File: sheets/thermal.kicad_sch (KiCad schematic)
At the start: 40 parts, among them U1 MAX31856, U3 MAX31856, U4 MAX31856, U5 MAX31856, U6 MAX31856, U7 MAX31856, U8 MAX31856, U9 MAX31856

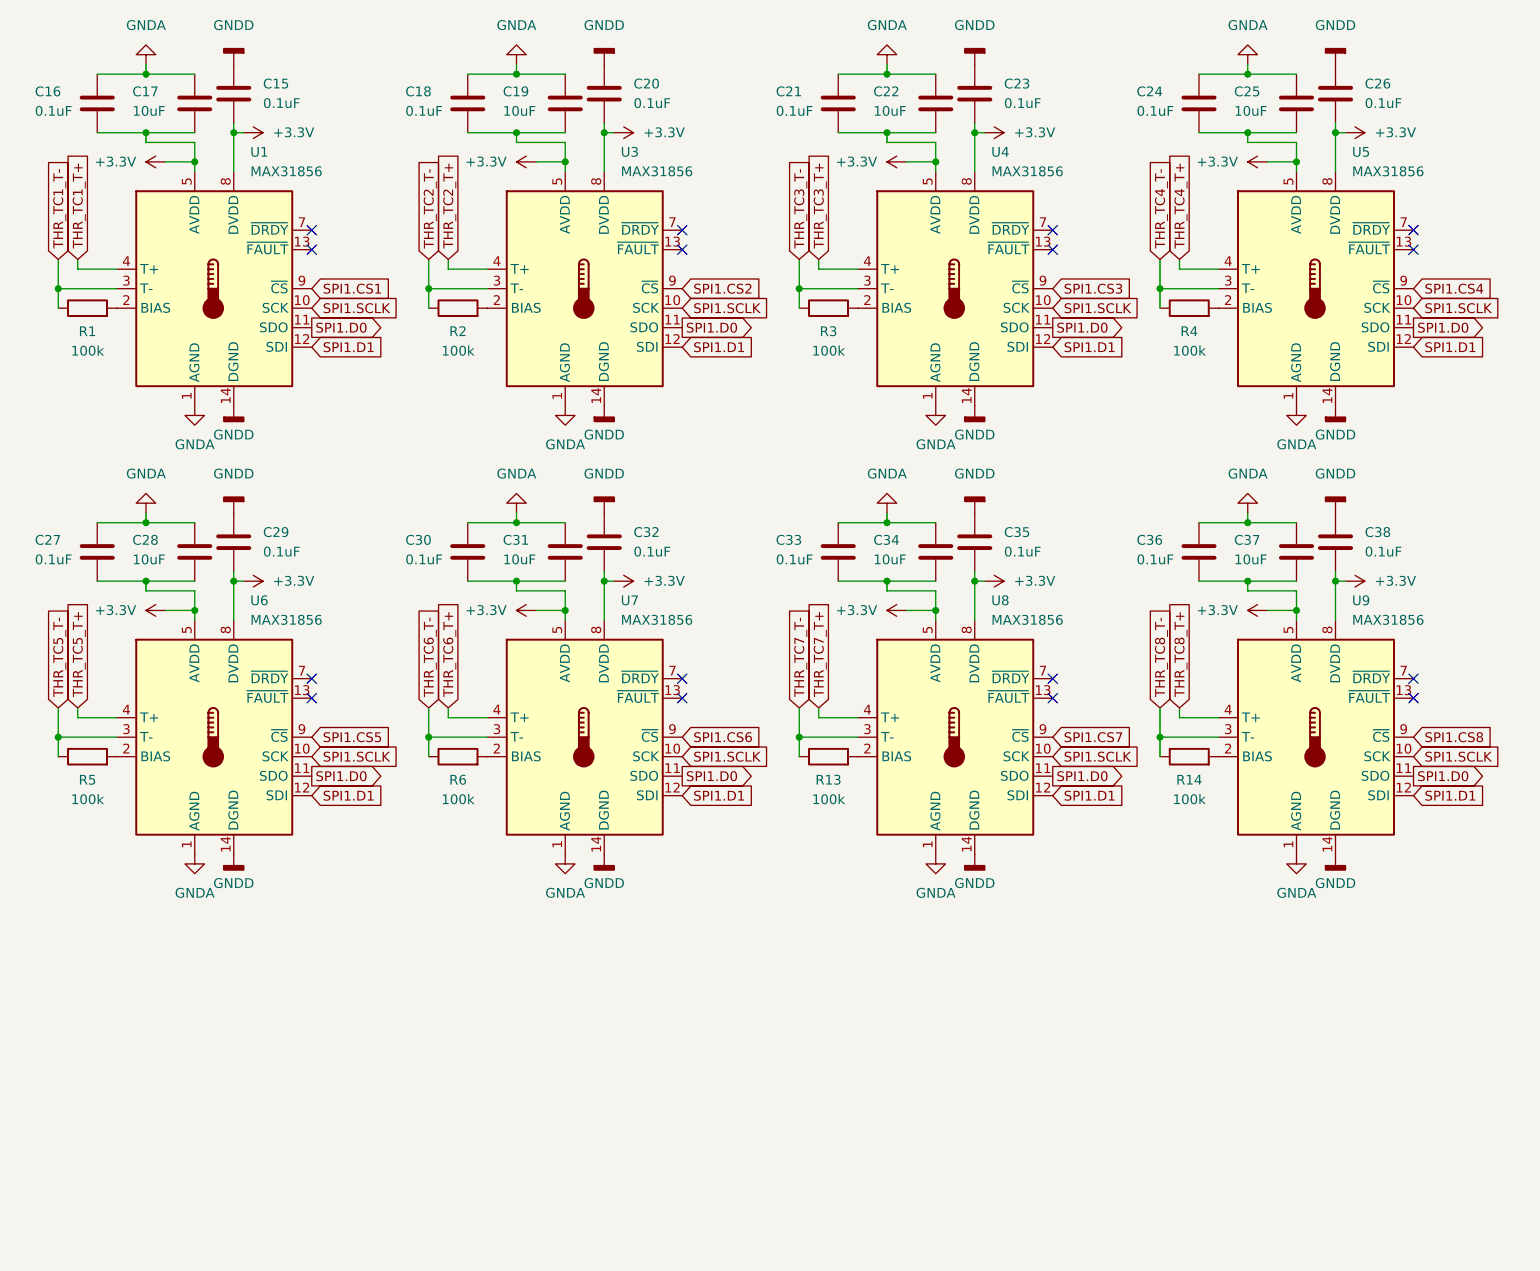
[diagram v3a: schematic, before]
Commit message: push
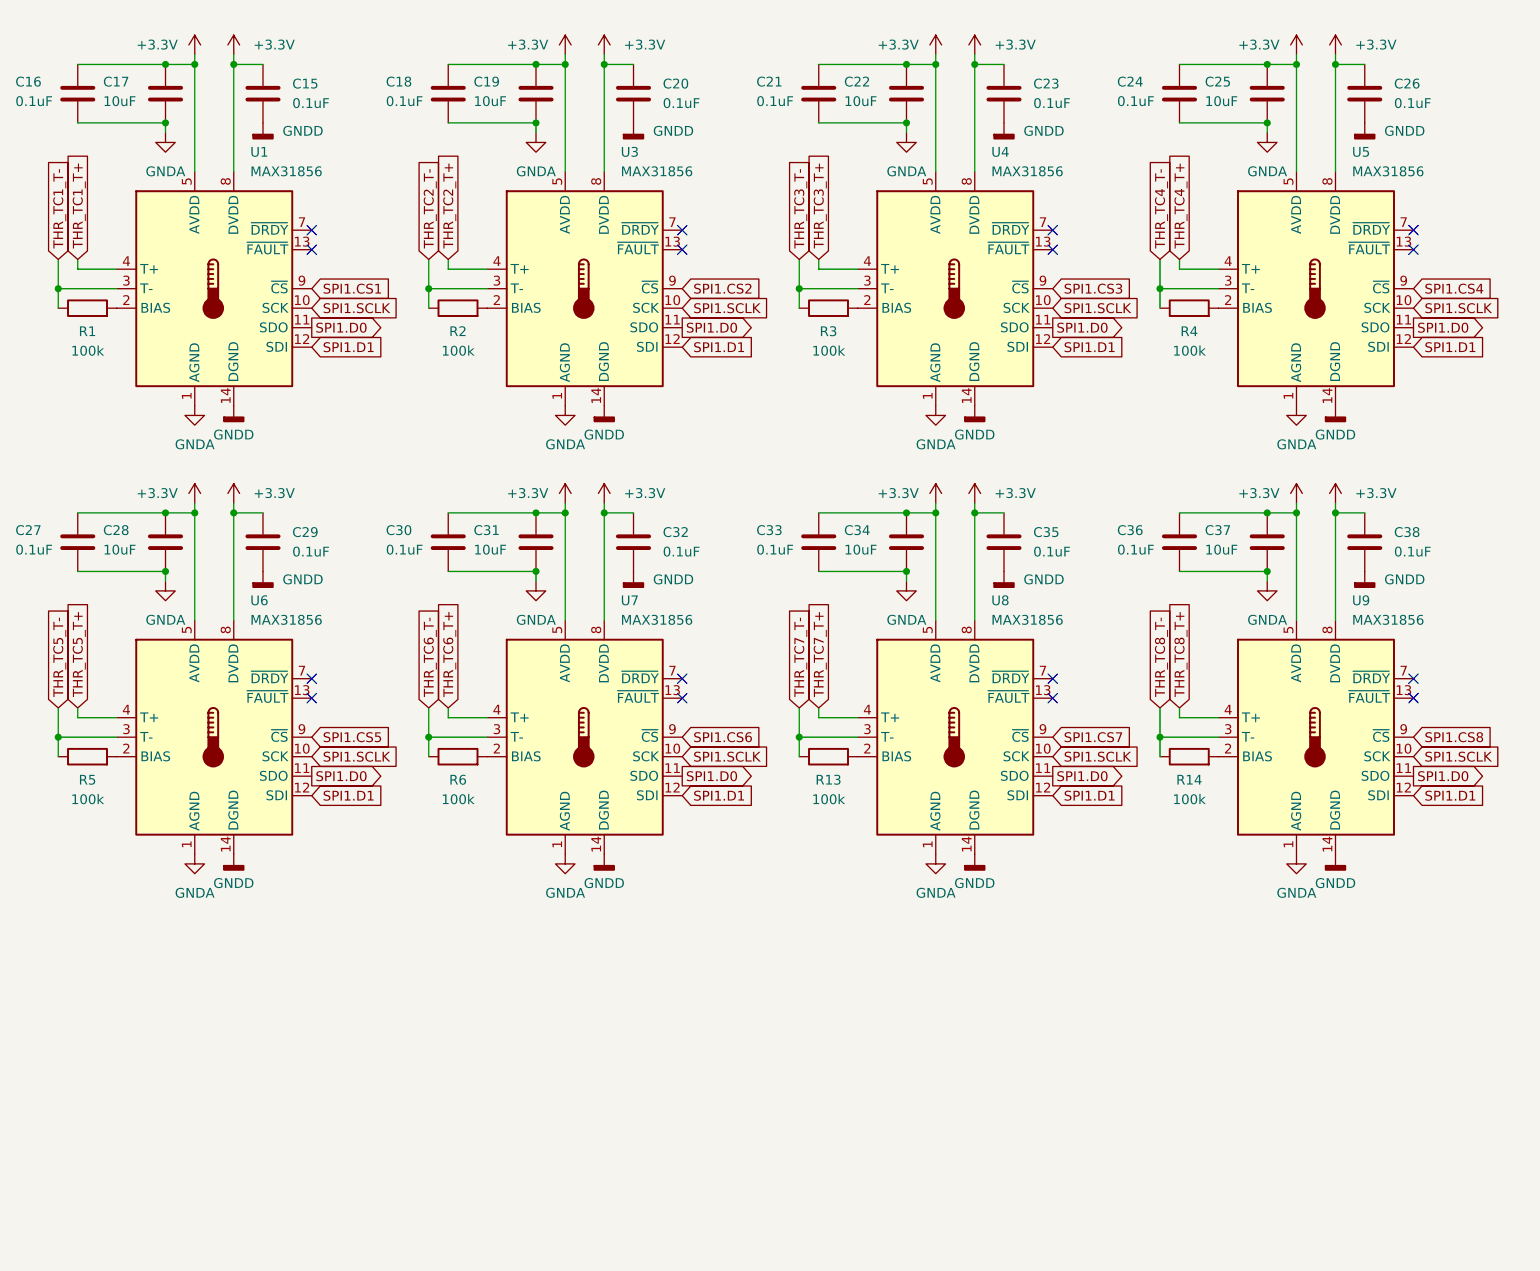
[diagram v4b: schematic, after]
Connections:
- net +3.3V: now also C15.1, C16.1, C17.1, C18.1, C19.1, C20.1, C21.1, C22.1, C23.1, C24.1, C25.1, C26.1, C27.1, C28.1, C29.1, C30.1, C31.1, C32.1, C33.1, C34.1, C35.1, C36.1, C37.1, C38.1; no longer C15.2, C16.2, C17.2, C18.2, C19.2, C20.2, C21.2, C22.2, C23.2, C24.2, C25.2, C26.2, C27.2, C28.2, C29.2, C30.2, C31.2, C32.2, C33.2, C34.2, C35.2, C36.2, C37.2, C38.2
- net GNDA: now also C16.2, C17.2, C18.2, C19.2, C21.2, C22.2, C24.2, C25.2, C27.2, C28.2, C30.2, C31.2, C33.2, C34.2, C36.2, C37.2; no longer C16.1, C17.1, C18.1, C19.1, C21.1, C22.1, C24.1, C25.1, C27.1, C28.1, C30.1, C31.1, C33.1, C34.1, C36.1, C37.1
- net GNDD: now also C15.2, C20.2, C23.2, C26.2, C29.2, C32.2, C35.2, C38.2; no longer C15.1, C20.1, C23.1, C26.1, C29.1, C32.1, C35.1, C38.1
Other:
- moved on the sheet: C15, C16, C17
